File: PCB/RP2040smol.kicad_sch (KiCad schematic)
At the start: 40 parts, among them SW1 BOOTSEL, SW2 RESET, U1 AP2112K-3.3, U2 RP2040, U3 W25Q64JVZP, Y1 Crystal_520-120-18-33JGN-TR3

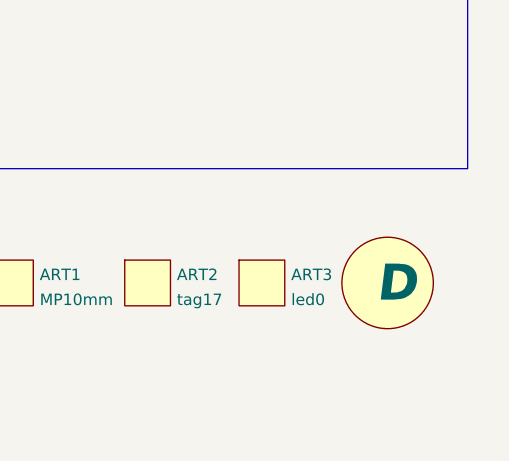
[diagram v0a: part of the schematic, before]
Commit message: E
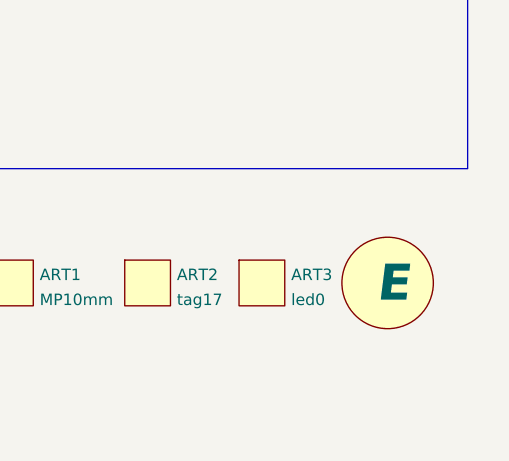
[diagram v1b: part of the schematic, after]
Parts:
- MISC1: value D -> E
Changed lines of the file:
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@@
       (effects (font (size 1.27 1.27)) hide)
     )
-    (property "Value" "D" (id 1) (at 274.32 173.99 0)
+    (property "Value" "E" (id 1) (at 274.32 173.99 0)
       (effects (font (size 4 4) bold italic) (justify left))
     )
@@
     )
     (path "/391dcbac-64b5-4436-a171-22510e2cc165"
-      (reference "MISC1") (unit 1) (value "D") (footprint "MikeFootprintLib:RevisionSymbol_Small")
+      (reference "MISC1") (unit 1) (value "E") (footprint "MikeFootprintLib:RevisionSymbol_Small")
     )
     (path "/6eeba014-e27c-49cf-b969-597642a973b0"
